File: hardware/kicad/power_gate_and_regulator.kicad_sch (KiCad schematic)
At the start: 12 parts, among them Q2 DMG3415U-7, Q2 PMV32UP, U4 XC6220, U5 TPL5110

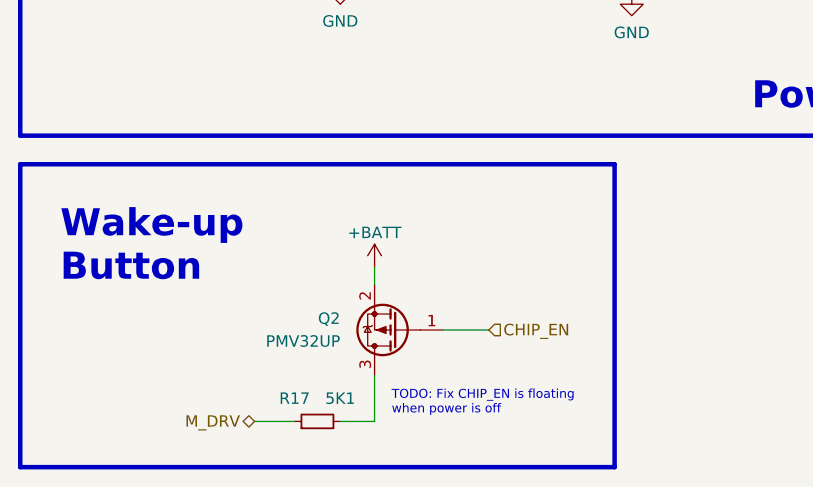
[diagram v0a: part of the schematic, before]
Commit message: wip wake-up button
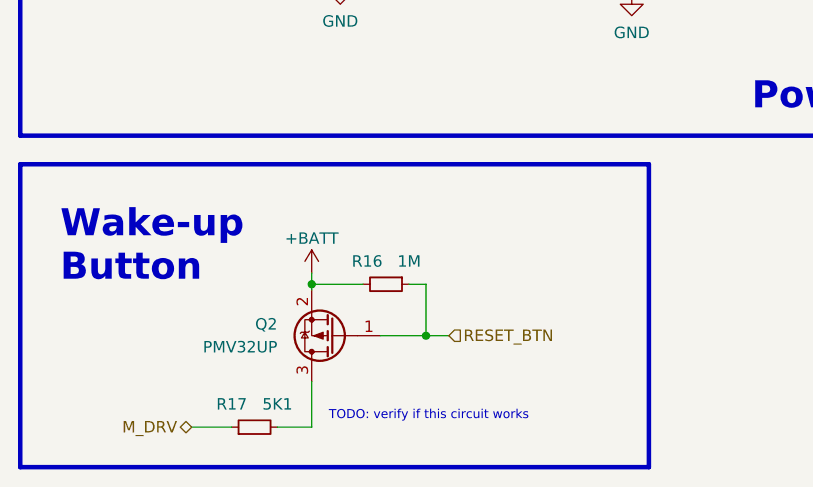
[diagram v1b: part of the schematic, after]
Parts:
- added R16: 1M, Resistor_SMD:R_0402_1005Metric, symbol Device:R_Small
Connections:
- net +BATT: now also R16.2
- net CHIP_EN renamed RESET_BTN
- net RESET_BTN: now also R16.1
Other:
- note added: "TODO: verify if this circuit works"
- note removed: "TODO: Fix CHIP_EN is floating when power is off"
- moved on the sheet: Q2, R17
